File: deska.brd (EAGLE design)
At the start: 25.7 x 40 mm, 11 parts

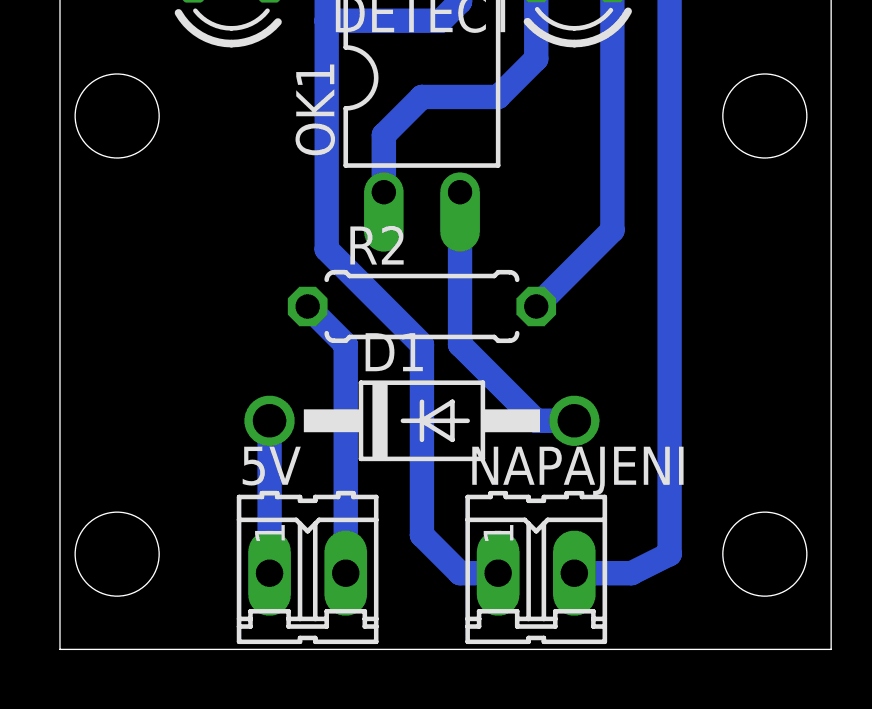
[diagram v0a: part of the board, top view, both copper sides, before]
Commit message: v0.3
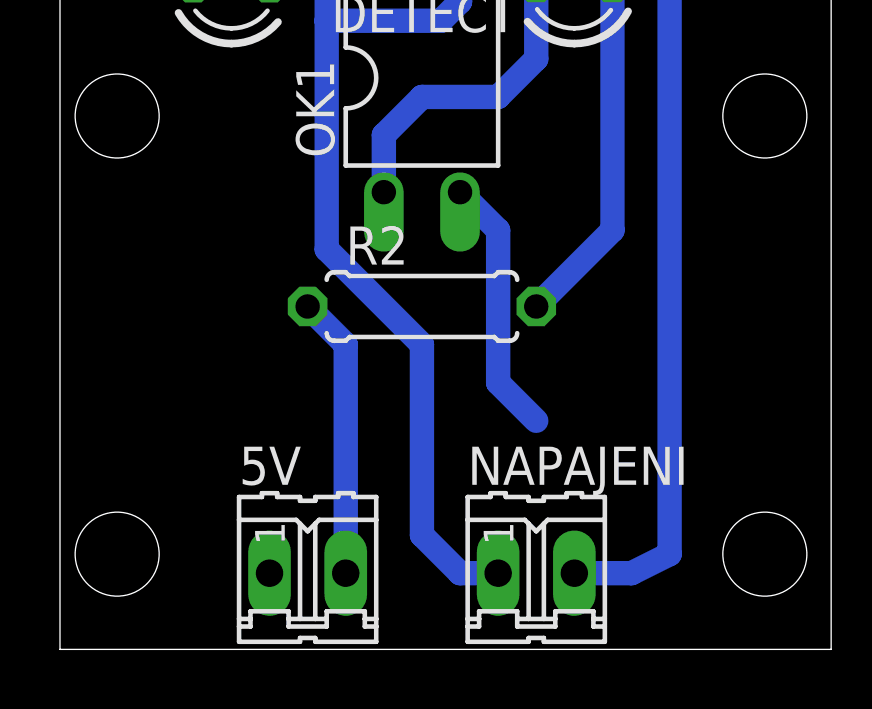
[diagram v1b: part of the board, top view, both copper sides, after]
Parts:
- removed D1: 1N4004, diode:DO41-10
- R4: value 1k -> 220
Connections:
- removed net N$4: 5V.1, D1.C
- net N$6: now also 5V.1; no longer D1.A
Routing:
- net N$4: track 5.08 -> 0.00 mm
- net N$6: track 9.94 -> 8.67 mm
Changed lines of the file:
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@@
 <attribute name="OC_NEWARK" value="unknown" x="8.255" y="2.54" size="1.778" layer="27" display="off"/>
 </element>
-<element name="D1" library="diode" package="DO41-10" value="1N4004" x="12.065" y="7.62"/>
 <element name="DETECT" library="led" package="LED3MM" value="" x="17.145" y="22.225" rot="R180"/>
 <element name="NAPAJENI" library="con-amp-quick" package="02P" value="" x="15.875" y="2.54">
@@
 <element name="R2" library="resistor" package="0207/7" value="1k" x="12.065" y="11.43"/>
 <element name="R3" library="resistor" package="0207/7" value="10k" x="12.065" y="33.02"/>
-<element name="R4" library="resistor" package="0207/7" value="1k" x="12.065" y="38.1"/>
+<element name="R4" library="resistor" package="0207/7" value="220" x="12.065" y="38.1"/>
 <element name="R5" library="resistor" package="0207/7" value="1k" x="12.065" y="35.56" rot="R180"/>
 <element name="STATUS" library="led" package="LED3MM" value="" x="5.715" y="22.225"/>
@@
 <wire x1="9.525" y1="2.54" x2="9.525" y2="10.16" width="0.8128" layer="16"/>
 <wire x1="9.525" y1="10.16" x2="8.255" y2="11.43" width="0.8128" layer="16"/>
-</signal>
-<signal name="N$4">
-<contactref element="5V" pad="1"/>
-<contactref element="D1" pad="C"/>
-<wire x1="6.985" y1="2.54" x2="6.985" y2="7.62" width="0.8128" layer="16"/>
 </signal>
 <signal name="GND">
@@
 <signal name="N$6">
 <contactref element="OK1" pad="2"/>
-<contactref element="D1" pad="A"/>
-<wire x1="13.335" y1="15.24" x2="13.335" y2="10.16" width="0.8128" layer="16"/>
-<wire x1="13.335" y1="10.16" x2="15.875" y2="7.62" width="0.8128" layer="16"/>
-<wire x1="15.875" y1="7.62" x2="17.145" y2="7.62" width="0.8128" layer="16"/>
+<wire x1="14.605" y1="13.97" x2="14.605" y2="8.89" width="0.8128" layer="16"/>
+<wire x1="14.605" y1="8.89" x2="15.875" y2="7.62" width="0.8128" layer="16"/>
+<contactref element="5V" pad="1"/>
+<wire x1="6.985" y1="2.54" x2="14.605" y2="8.89" width="0" layer="19" extent="16-16"/>
+<wire x1="13.335" y1="15.24" x2="14.605" y2="13.97" width="0.8128" layer="16"/>
 </signal>
 </signals>
